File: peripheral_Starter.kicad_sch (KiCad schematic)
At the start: 51 parts, among them J1 Conn_01x04_Pin, J10 Conn_01x05, J11 Conn_01x05, J2 Conn_01x03_Pin, J3 Conn_01x04_Pin, J4 Conn_01x06_Pin, J5 Conn_01x02_Pin, J6 Conn_01x02_Pin, J7 Conn_01x02_Pin, J8 Conn_01x04_Pin, J9 Conn_01x02_Pin, Q1 BC547, SW1 SW_Push, SW2 SW_Push, SW3 SW_Push, SW4 SW_Push, SW5 Slide Sw, U1 AMS1117-3.3

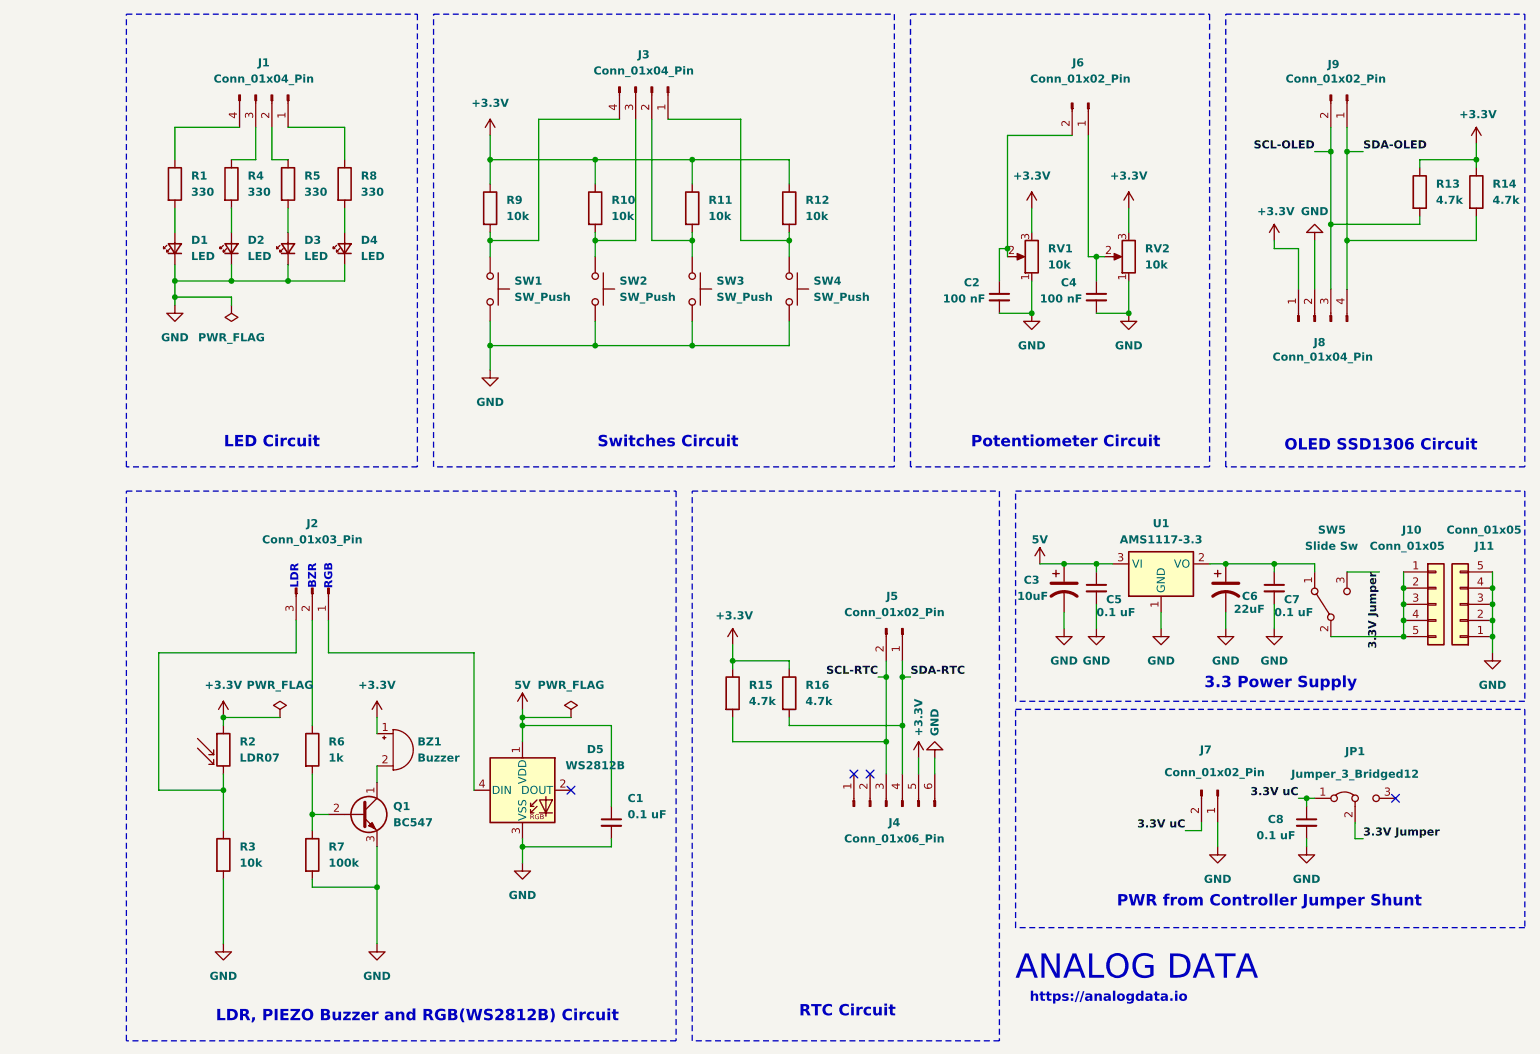
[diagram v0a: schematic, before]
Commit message: Power Section Added and Sheets Updated
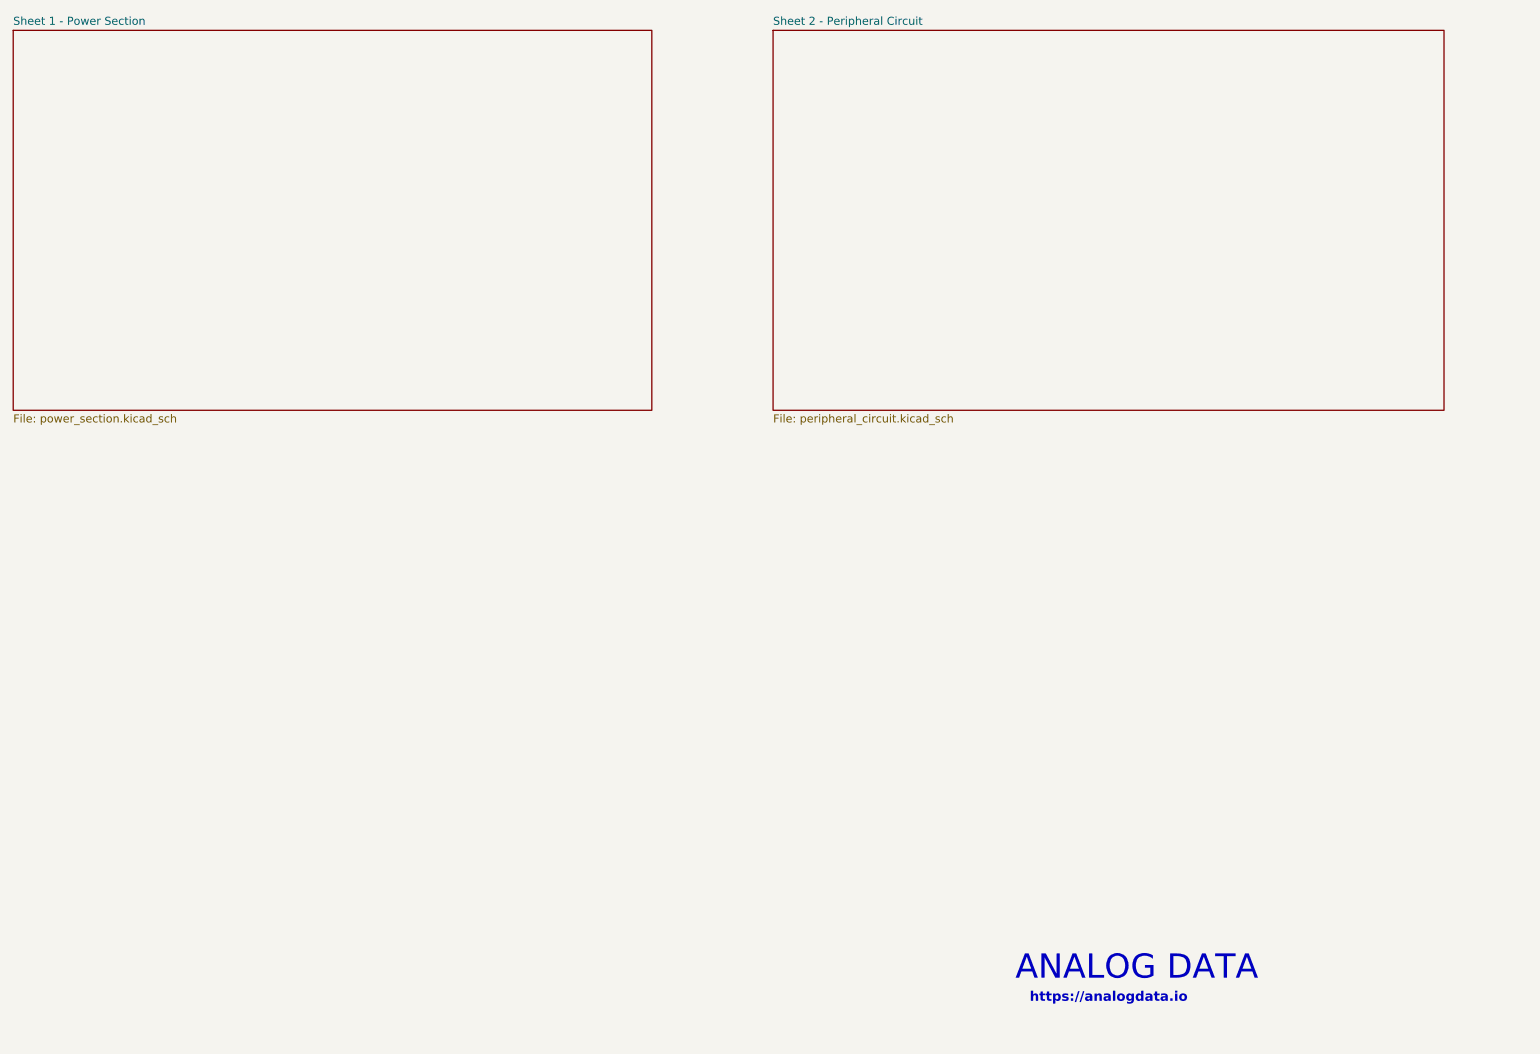
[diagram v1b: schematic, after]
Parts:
- removed BZ1: Buzzer, symbol Device:Buzzer
- removed C1, C5, C7, C8: 0.1 uF, PCM_SparkFun-Capacitor:C_0603_1608Metric, symbol PCM_SparkFun-Capacitor:C
- removed C2, C4: 100 nF, PCM_SparkFun-Capacitor:C_0603_1608Metric, symbol PCM_SparkFun-Capacitor:C
- removed C3: 10uF, Capacitor_THT:CP_Radial_D13.0mm_P5.00mm, symbol PCM_SparkFun-Capacitor:C_Polarized
- removed C6: 22uF, Capacitor_THT:CP_Radial_D14.0mm_P5.00mm, symbol PCM_SparkFun-Capacitor:C_Polarized
- removed D1, D2, D3, D4: LED, PCM_SparkFun-LED:LED_0603_1608Metric, symbol PCM_SparkFun-LED:LED
- removed D5: WS2812B, LED_SMD:LED_WS2812B_PLCC4_5.0x5.0mm_P3.2mm, symbol LED:WS2812B
- removed J1, J3, J8: Conn_01x04_Pin, symbol Connector:Conn_01x04_Pin
- removed J10, J11: Conn_01x05, symbol Connector_Generic:Conn_01x05
- removed J2: Conn_01x03_Pin, symbol Connector:Conn_01x03_Pin
- removed J4: Conn_01x06_Pin, symbol Connector:Conn_01x06_Pin
- removed J5, J6, J7, J9: Conn_01x02_Pin, symbol Connector:Conn_01x02_Pin
- removed JP1: Jumper_3_Bridged12, symbol Jumper:Jumper_3_Bridged12
- removed Q1: BC547, Package_TO_SOT_THT:TO-92_Inline, symbol Transistor_BJT:BC547
- removed R1, R4, R5, R8: 330, symbol Device:R
- removed R10, R11, R12, R3, R9: 10k, symbol Device:R
- removed R13, R14, R15, R16: 4.7k, symbol Device:R
- removed R2: LDR07, OptoDevice:R_LDR_5.1x4.3mm_P3.4mm_Vertical, symbol Sensor_Optical:LDR07
- removed R6: 1k, symbol Device:R
- removed R7: 100k, symbol Device:R
- removed RV1, RV2: 10k, symbol Device:R_Potentiometer
- removed SW1, SW2, SW3, SW4: SW_Push, symbol Switch:SW_Push
- removed SW5: Slide Sw, PCM_SparkFun-Switch:Slide_SPDT_PTH_11.6x4.0mm, symbol PCM_SparkFun-Switch:SPDT_Slide_PTH_11.6x4.0mm
- removed U1: AMS1117-3.3, Package_TO_SOT_SMD:SOT-223-3_TabPin2, symbol Regulator_Linear:AMS1117-3.3
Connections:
- no-connect marks 4 -> 0
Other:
- added sheet Sheet 1 - Power Section (power_section.kicad_sch)
- added sheet Sheet 2 - Peripheral Circuit (peripheral_circuit.kicad_sch)
- note removed: "3.3 Power Supply"
- note removed: "BZR"
- note removed: "LDR"
- note removed: "LDR, PIEZO Buzzer and RGB(WS2812B) Circuit"
- note removed: "LED Circuit"
- note removed: "OLED SSD1306 Circuit"
- note removed: "PWR from Controller Jumper Shunt"
- note removed: "Potentiometer Circuit"
- note removed: "RGB"
- note removed: "RTC Circuit"
- note removed: "Switches Circuit"
